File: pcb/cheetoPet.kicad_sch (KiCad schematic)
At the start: 46 parts, among them J1 SH1107 Display 128x128, P1 USB_C_Plug_USB2.0, SW1 B, SW2 X, SW3 A, SW4 POWER, SW5 RESET, SW6 BOOT, U1 DS3231M, U2 MPU-9250, U3 TP4056-42-ESOP8, U4 ESP32-C3-WROOM-02U, U5 ADS1115IDGS, U6 TPS63802DLAR, U7 AT24CS04-SSHM

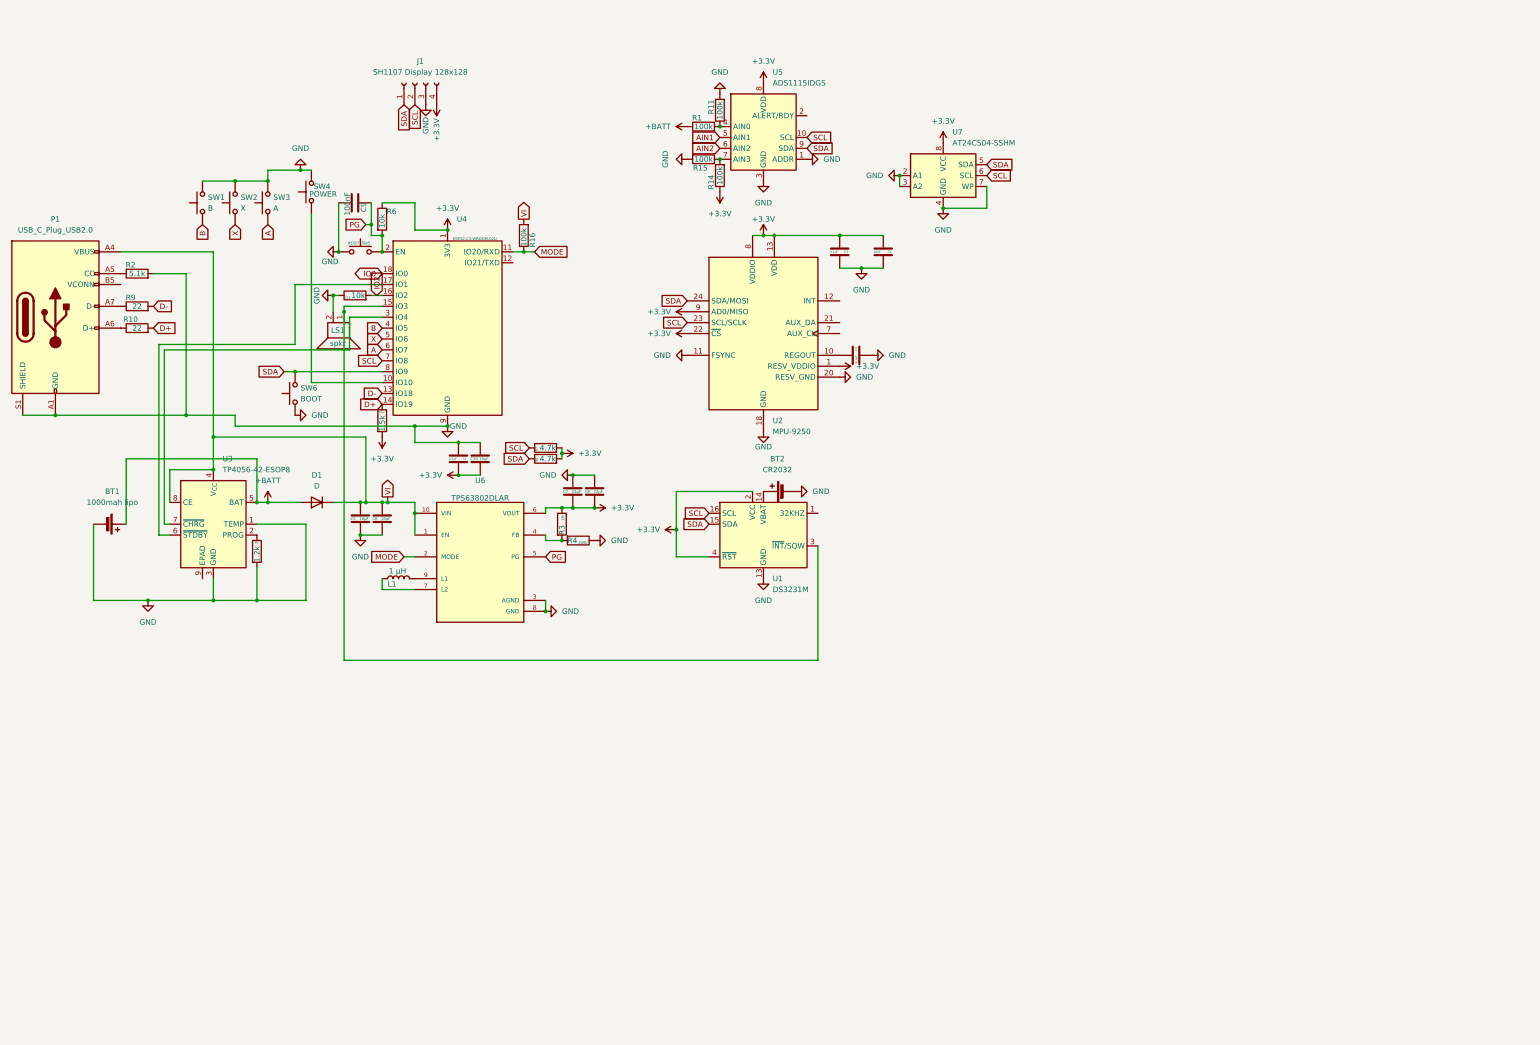
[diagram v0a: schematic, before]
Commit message: new pcb lol
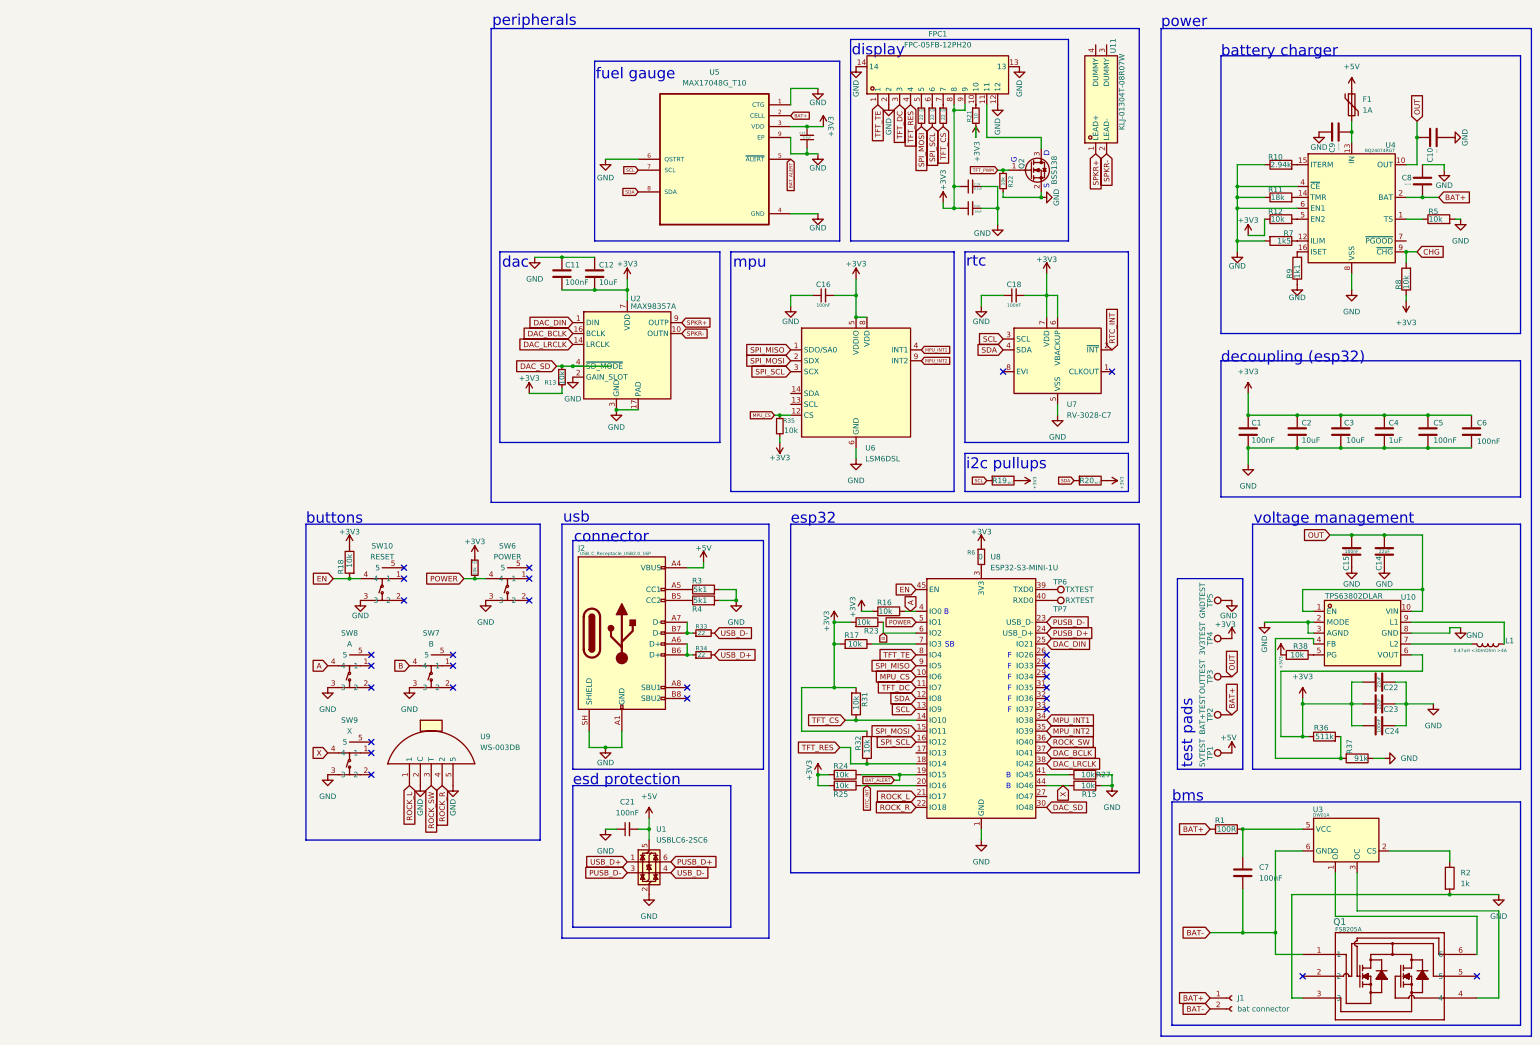
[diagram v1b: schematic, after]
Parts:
- removed BT1: 1000mah lipo, Connector_PinHeader_2.54mm:PinHeader_1x02_P2.54mm_Vertical, symbol Device:Battery_Cell
- removed BT2: CR2032, Connector_PinHeader_2.54mm:PinHeader_1x02_P2.54mm_Vertical, symbol Device:Battery_Cell
- removed D1: D, Diode_SMD:D_0805_2012Metric_Pad1.15x1.40mm_HandSolder, symbol Device:D
- removed J1: SH1107 Display 128x128, Connector_PinHeader_2.54mm:PinHeader_1x04_P2.54mm_Vertical, symbol Connector:Conn_01x04_Socket
- removed LS1: spkr, cheeto:PS1240_PassiveBuzzer_12.2x3.5mm, symbol Device:Speaker
- removed P1: USB_C_Plug_USB2.0, Connector_USB:USB_C_Receptacle_HRO_TYPE-C-31-M-12, symbol Connector:USB_C_Plug_USB2.0
- removed R13, R6: 10k, Resistor_SMD:R_0805_2012Metric_Pad1.20x1.40mm_HandSolder, symbol Device:R
- removed R14: 100k, Resistor_SMD:R_0805_2012Metric_Pad1.20x1.40mm_HandSolder, symbol Device:R
- removed SW1: B, Library:PushButton_SMD_3_4_2mm, symbol Switch:SW_Push
- removed SW2: X, Library:PushButton_SMD_3_4_2mm, symbol Switch:SW_Push
- removed SW3: A, Library:PushButton_SMD_3_4_2mm, symbol Switch:SW_Push
- removed SW4: POWER, cheeto:side switch, symbol Switch:SW_Push
- removed SW5: RESET, Library:PushButton_SMD_3_4_2mm, symbol Switch:SW_Push
- removed SW6: BOOT, Library:PushButton_SMD_3_4_2mm, symbol Switch:SW_Push
- removed U1: DS3231M, Package_SO:SOIC-16W_7.5x10.3mm_P1.27mm, symbol Timer_RTC:DS3231M
- removed U2: MPU-9250, Sensor_Motion:InvenSense_QFN-24_3x3mm_P0.4mm, symbol Sensor_Motion:MPU-9250
- removed U3: TP4056-42-ESOP8, Package_SO:SOIC-8-1EP_3.9x4.9mm_P1.27mm_EP2.41x3.3mm_ThermalVias, symbol Battery_Management:TP4056-42-ESOP8
- removed U4: ESP32-C3-WROOM-02U, RF_Module:ESP32-C3-WROOM-02U, symbol RF_Module:ESP32-C3-WROOM-02U
- removed U5: ADS1115IDGS, Package_SO:TSSOP-10_3x3mm_P0.5mm, symbol Analog_ADC:ADS1115IDGS
- removed U6: TPS63802DLAR, cheeto:VREG_TPS63802DLAR, symbol cheeto:TPS63802DLAR
- removed U7: AT24CS04-SSHM, Package_SO:SOIC-8_3.9x4.9mm_P1.27mm, symbol Memory_EEPROM:AT24CS04-SSHM
- added C11: 100nF, Capacitor_SMD:C_0402_1005Metric, symbol Device:C
- added C12: 10uF, Capacitor_SMD:C_0603_1608Metric, symbol Device:C
- added C14, C22, C23: 22uF, Capacitor_SMD:C_0805_2012Metric, symbol Device:C
- added C15, C24: 100nF, Capacitor_SMD:C_0603_1608Metric, symbol Device:C
- added C16, C18, C21: 100nF, Capacitor_SMD:C_0603_1608Metric, symbol Device:C_Small
- added C17, C19: 0.1uF, Capacitor_SMD:C_0402_1005Metric, symbol Device:C_Small
- added C20: 10uF, Capacitor_SMD:C_0603_1608Metric, symbol Device:C_Small
- added F1: 1A, Fuse:Fuse_1812_4532Metric, symbol Device:Polyfuse
- added FPC1: FPC-05FB-12PH20, EasyEDA:FPC-SMD_12P-P0.50_XUNPU_FPC-05FB-12PH20, symbol EasyEDA:FPC-05FB-12PH20
- added J1: bat connector, Connector_PinHeader_2.00mm:PinHeader_1x02_P2.00mm_Vertical, symbol Connector:Conn_01x02_Socket
- added J2: USB_C_Receptacle_USB2.0_16P, Connector_USB:USB_C_Receptacle_G-Switch_GT-USB-7010ASV, symbol Connector:USB_C_Receptacle_USB2.0_16P
- added Q1: FS8205A, footprints:SOT-23-6L_TCP, symbol 2026-06-26_17-03-40:FS8205A
- added Q2: BSS138, Package_TO_SOT_SMD:SOT-23, symbol Transistor_FET:BSS138
- added R13, R22, R26, R35: 10k, Resistor_SMD:R_0402_1005Metric, symbol Device:R_Small
- added R17, R18, R23, R24, R25, R27, R31, R32, R38: 10k, Resistor_SMD:R_0402_1005Metric, symbol Device:R
- added R19, R20: 4k7, Resistor_SMD:R_0402_1005Metric, symbol Device:R
- added R21: 10, Resistor_SMD:R_0402_1005Metric, symbol Device:R_Small
- added R28, R29, R30, R33, R34: 22, Resistor_SMD:R_0402_1005Metric, symbol Device:R_Small
- added R36: 511k, Resistor_SMD:R_0402_1005Metric, symbol Device:R
- added R37: 91k, Resistor_SMD:R_0402_1005Metric, symbol Device:R
- added R6: 0, Resistor_SMD:R_0402_1005Metric, symbol Device:R_Small
- added SW10: RESET, EasyEDA:SW-SMD_5P-L4.2-W2.8-P1.60-LS4.6-TR, symbol EasyEDA:KMR223GLFG
- added SW6: POWER, EasyEDA:SW-SMD_5P-L4.2-W2.8-P1.60-LS4.6-TR, symbol EasyEDA:KMR223GLFG
- added SW7: B, EasyEDA:SW-SMD_5P-L4.2-W2.8-P1.60-LS4.6-TR, symbol EasyEDA:KMR223GLFG
- added SW8: A, EasyEDA:SW-SMD_5P-L4.2-W2.8-P1.60-LS4.6-TR, symbol EasyEDA:KMR223GLFG
- added SW9: X, EasyEDA:SW-SMD_5P-L4.2-W2.8-P1.60-LS4.6-TR, symbol EasyEDA:KMR223GLFG
- added TP1: 5VTEST, TestPoint:TestPoint_Pad_1.5x1.5mm, symbol Connector:TestPoint
- added TP2: BAT+TEST, TestPoint:TestPoint_Pad_1.5x1.5mm, symbol Connector:TestPoint
- added TP3: OUTTEST, TestPoint:TestPoint_Pad_1.5x1.5mm, symbol Connector:TestPoint
- added TP4: 3V3TEST, TestPoint:TestPoint_Pad_1.5x1.5mm, symbol Connector:TestPoint
- added TP5: GNDTEST, TestPoint:TestPoint_Pad_1.5x1.5mm, symbol Connector:TestPoint
- added TP6: TXTEST, TestPoint:TestPoint_Pad_1.5x1.5mm, symbol Connector:TestPoint
- added TP7: RXTEST, TestPoint:TestPoint_Pad_1.5x1.5mm, symbol Connector:TestPoint
- added U1: USBLC6-2SC6, Package_TO_SOT_SMD:SOT-23-6, symbol Power_Protection:USBLC6-2SC6
- added U10: TPS63802DLAR, EasyEDA:VSON-10_L3.0-W2.0-P0.50-TL, symbol EasyEDA:TPS63802DLAR
- added U11: KLJ-01304T-08R07W, EasyEDA:BUZ-SMD_4P-L13.0-W13.0-P11.4-BL, symbol EasyEDA:KLJ-01304T-08R07W
- added U2: MAX98357A, Package_DFN_QFN:TQFN-16-1EP_3x3mm_P0.5mm_EP1.23x1.23mm, symbol Audio:MAX98357A
- added U3: DW01A, Package_TO_SOT_SMD:SOT-23-6, symbol Battery_Management:DW01A
- added U4: BQ24074RGT, Package_DFN_QFN:VQFN-16-1EP_3x3mm_P0.5mm_EP1.6x1.6mm, symbol Battery_Management:BQ24074RGT
- added U5: MAX17048G_T10, MAX17048G_T10:SON50P200X200X80-9N, symbol MAX17048G_T10:MAX17048G_T10
- added U6: LSM6DSL, Package_LGA:LGA-14_3x2.5mm_P0.5mm_LayoutBorder3x4y, symbol Sensor_Motion:LSM6DSL
- added U7: RV-3028-C7, Package_SON:MicroCrystal_C7_SON-8_1.5x3.2mm_P0.9mm, symbol Timer_RTC:RV-3028-C7
- added U8: ESP32-S3-MINI-1U, RF_Module:ESP32-S2-MINI-1U, symbol RF_Module:ESP32-S3-MINI-1U
- added U9: WS-003DB, EasyEDA:SW-SMD_WS-003DB, symbol EasyEDA:WS-003DB
- C1: value 0.1µF -> 100nF; footprint Capacitor_SMD:C_0805_2012Metric_Pad1.18x1.45mm_HandSolder -> Capacitor_SMD:C_0402_1005Metric
- C10: value 10µF -> 22uF; footprint Capacitor_SMD:C_0805_2012Metric_Pad1.18x1.45mm_HandSolder -> Capacitor_SMD:C_0805_2012Metric
- C2: value 0.1µf -> 10uF; footprint Capacitor_SMD:C_0805_2012Metric_Pad1.18x1.45mm_HandSolder -> Capacitor_SMD:C_0603_1608Metric
- C3: value 0.1uF -> 10uF; footprint Capacitor_SMD:C_0805_2012Metric_Pad1.18x1.45mm_HandSolder -> Capacitor_SMD:C_0603_1608Metric
- C4: value 10uF -> 1uF; footprint Capacitor_SMD:C_0805_2012Metric_Pad1.18x1.45mm_HandSolder -> Capacitor_SMD:C_0402_1005Metric
- C5, C6: value 10µF -> 100nF; footprint Capacitor_SMD:C_0805_2012Metric_Pad1.18x1.45mm_HandSolder -> Capacitor_SMD:C_0402_1005Metric
- C7: value 22µF -> 100nF; footprint Capacitor_SMD:C_0805_2012Metric_Pad1.18x1.45mm_HandSolder -> Capacitor_SMD:C_0402_1005Metric
- C8: value 22µF -> 10uF X5R; footprint Capacitor_SMD:C_0805_2012Metric_Pad1.18x1.45mm_HandSolder -> Capacitor_SMD:C_0603_1608Metric
- C9: value 100nF -> 10uF X5R; footprint Capacitor_SMD:C_0603_1608Metric_Pad1.08x0.95mm_HandSolder -> Capacitor_SMD:C_0603_1608Metric
- L1: value 1 µH -> 0.47uH <30mOhm >4A; footprint Inductor_SMD:L_Changjiang_FXL0420 -> EasyEDA:L1008
- R1: value 100k -> 100R; footprint Resistor_SMD:R_0805_2012Metric_Pad1.20x1.40mm_HandSolder -> Resistor_SMD:R_0402_1005Metric
- R10: value 22 -> 2.94k; footprint Resistor_SMD:R_0805_2012Metric_Pad1.20x1.40mm_HandSolder -> Resistor_SMD:R_0402_1005Metric
- R11: value 100k -> 18k; footprint Resistor_SMD:R_0805_2012Metric_Pad1.20x1.40mm_HandSolder -> Resistor_SMD:R_0402_1005Metric
- R12: value 1.5k -> 10k; footprint Resistor_SMD:R_0805_2012Metric_Pad1.20x1.40mm_HandSolder -> Resistor_SMD:R_0402_1005Metric
- R15, R16: value 100k -> 10k; footprint Resistor_SMD:R_0805_2012Metric_Pad1.20x1.40mm_HandSolder -> Resistor_SMD:R_0402_1005Metric
- R2: value 5.1k -> 1k; footprint Resistor_SMD:R_0805_2012Metric_Pad1.20x1.40mm_HandSolder -> Resistor_SMD:R_0402_1005Metric
- R3: value 1M -> 5k1; footprint Resistor_SMD:R_1206_3216Metric_Pad1.30x1.75mm_HandSolder -> Resistor_SMD:R_0402_1005Metric
- R4: value 309k -> 5k1; footprint Resistor_SMD:R_0402_1005Metric_Pad0.72x0.64mm_HandSolder -> Resistor_SMD:R_0402_1005Metric
- R5: value 1.2k -> 10k; footprint Resistor_SMD:R_0805_2012Metric_Pad1.20x1.40mm_HandSolder -> Resistor_SMD:R_0402_1005Metric
- R7: value 4.7k -> 1k5; footprint Resistor_SMD:R_0805_2012Metric_Pad1.20x1.40mm_HandSolder -> Resistor_SMD:R_0402_1005Metric
- R8: value 4.7k -> 10k; footprint Resistor_SMD:R_0805_2012Metric_Pad1.20x1.40mm_HandSolder -> Resistor_SMD:R_0402_1005Metric
- R9: value 22 -> 1k1; footprint Resistor_SMD:R_0805_2012Metric_Pad1.20x1.40mm_HandSolder -> Resistor_SMD:R_0402_1005Metric
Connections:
- net MODE is gone; now on net A: R16.1
- net VI is gone; now on net +3V3: C5.1, C6.1, R16.2
- net A: now also SW8.4, U8.4 (IO0)
- net B: now also R23.1, SW7.4, U8.6 (IO2)
- net GND: now also C1.2, C10.2, R10.1, R11.1, R3.2, R4.2, R7.2, R9.1, C11.1, C12.1, C14.2, C15.2, C16.1, C17.1, C18.1, C19.2, C20.2, C21.1, C22.2, C23.2, C24.2, FPC1.12, FPC1.13, FPC1.14, FPC1.2, J2.A1 (GND), J2.A12 (GND), J2.B1 (GND), J2.B12 (GND), J2.SH (SHIELD), Q1.3, Q2.2 (S), R22.2, R27.2, R37.1, SW10.3, SW6.3, SW7.3, SW8.3, SW9.3, TP5.1, U1.2 (GND), U10.2 (MODE), U10.3 (AGND), U10.8 (GND), U2.11 (GND), U2.15 (GND), U2.17 (PAD), U2.2 (GAIN_SLOT), U2.3 (GND), U4.17 (VSS), U4.4 (~{CE}), U4.6 (EN1), U4.8 (VSS), U5.1 (CTG), U5.4 (GND), U5.6 (QSTRT), U5.9 (EP), U6.6 (GND), U6.7 (GND), U7.5 (VSS), U8.1 (GND), U8.2 (GND), U8.42 (GND), U8.43 (GND), U8.46 (GND), U8.47 (GND), U8.48 (GND), U8.49 (GND), U8.50 (GND), U8.51 (GND), U8.52 (GND), U8.53 (GND), U8.54 (GND), U8.55 (GND), U8.56 (GND), U8.57 (GND), U8.58 (GND), U8.59 (GND), U8.60 (GND), U8.61 (GND), U8.62 (GND), U8.63 (GND), U8.64 (GND), U8.65 (GND), U9.2 (C), U9.5; no longer C1.1, C10.1, C7.1, R11.2, R4.1
- net SCL: now also R19.2, U5.7 (SCL), U7.3 (SCL), U8.13 (IO9); no longer R7.1
- net SDA: now also R20.2, U5.8 (SDA), U7.4 (SDA), U8.12 (IO8); no longer R8.1
- net X: now also R15.1, SW9.4, U8.44 (IO46)
- net +3V3: now reaches C2.1
- net +3V3: now also C1.1, C3.1, C4.1, R12.1, R8.1, C11.2, C12.2, C16.2, C17.2, C18.2, C19.1, C20.1, C22.1, C23.1, C24.1, FPC1.8, FPC1.9, R13.2, R17.2, R18.1, R19.1, R20.1, R21.2, R23.2, R24.2, R25.2, R26.1, R31.2, R32.2, R35.2, R36.1, R38.2, R6.1, TP4.1, U10.6 (VOUT), U2.7 (VDD), U2.8 (VDD), U5.3 (VDD), U6.5 (VDDIO), U6.8 (VDD), U7.6 (VBACKUP), U7.7 (VDD)
- net at R2.1: now also U3.2 (CS)
- net at R1.2: now also C7.1, U3.5 (VCC); no longer R11.1
- net at L1.1: now also U10.7 (L2)
- net at L1.2: now also U10.9 (L1)
- net at R5.1: now also U4.1 (TS)
- removed net +3.3V: C1.2, C10.2, C3.1, C4.1, C7.2, C8.2, R12.2, R3.1, R7.2, R8.2
- net +BATT renamed BAT+
- net BAT+: now also C8.2, J1.1 (Pin_1), TP2.1, U4.2 (BAT), U4.3 (BAT), U5.2 (CELL)
- net D+: no longer names the net of R10.2
- net D+: now also U4.15 (ITERM); no longer R12.1
- net D-: no longer names the net of R9.2
- net D-: now also U4.16 (ISET)
- net PG: no longer names the net of C9.2
- net PG: now also F1.2, U4.13 (IN)
- new net: R36.2, R37.2, U10.4 (FB)
- new net: FPC1.10, R21.1
- new net: FPC1.11, Q2.3 (D)
- new net: FPC1.5, R29.1
- new net: FPC1.6, R28.1
- new net: FPC1.7, R30.1
- new net: R7.1, U4.12 (ILIM)
- new net: R11.2, U4.14 (TMR)
- new net: R12.2, U4.5 (EN2)
- new net: TP6.1, U8.39 (TXD0)
- new net: R38.1, U10.5 (PG)
- new net: R17.1, U8.7 (IO3)
- new net: R27.1, U8.41 (IO45)
- new net: J2.A5 (CC1), R3.1
- new net: Q1.6, U3.1 (OD)
- new net: Q1.4, U3.3 (OC)
- new net: J2.A6 (D+), J2.B6 (D+), R34.1
- new net: J2.A7 (D-), J2.B7 (D-), R33.1
- new net: J2.B5 (CC2), R4.1
- new net: R6.2, U8.3 (3V3)
- new net: TP7.1, U8.40 (RXD0)
- new net +5V: C21.2, F1.1, J2.A4 (VBUS), J2.A9 (VBUS), J2.B4 (VBUS), J2.B9 (VBUS), TP1.1, U1.5 (VBUS)
- new net BAT-: C7.2, J1.2 (Pin_2), Q1.1, U3.6 (GND)
- new net BAT_ALERT: R24.1, U5.5 (~{ALERT}), U8.19 (IO15)
- new net CHG: R8.2, U4.9 (~{CHG})
- new net DAC_BCLK: U2.16 (BCLK), U8.37 (IO41)
- new net DAC_DIN: U2.1 (DIN), U8.25 (IO21)
- new net DAC_LRCLK: U2.14 (LRCLK), U8.38 (IO42)
- new net DAC_SD: R13.1, U2.4 (~{SD_MODE}), U8.30 (IO48)
- new net EN: R18.2, SW10.4, U8.45 (EN)
- new net MPU_CS: R35.1, U6.12 (CS), U8.10 (IO6)
- new net MPU_INT1: U6.4 (INT1), U8.34 (IO38)
- new net MPU_INT2: U6.9 (INT2), U8.35 (IO39)
- new net OUT: C10.1, C14.1, C15.1, TP3.1, U10.1 (EN), U10.10 (VIN), U4.10 (OUT), U4.11 (OUT)
- new net POWER: R26.2, SW6.4, U8.5 (IO1)
- new net PUSB_D+: U1.6 (I/O1), U8.24 (USB_D+)
- new net PUSB_D-: U1.3 (I/O2), U8.23 (USB_D-)
- new net ROCK_L: U8.21 (IO17), U9.1
- new net ROCK_R: U8.22 (IO18), U9.4 (2)
- new net ROCK_SW: U8.36 (IO40), U9.3 (T)
- new net RTC_INT: R25.1, U7.2 (~{INT}), U8.20 (IO16)
- new net SPI_MISO: U6.1 (SDO/SA0), U8.9 (IO5)
- new net SPI_MOSI: R29.2, U6.2 (SDX), U8.15 (IO11)
- new net SPI_SCL: R28.2, U6.3 (SCX), U8.16 (IO12)
- new net SPKR+: U11.1 (LEAD+), U2.9 (OUTP)
- new net SPKR-: U11.2 (LEAD-), U2.10 (OUTN)
- new net TFT_CS: R30.2, R31.1, U8.14 (IO10)
- new net TFT_DC: FPC1.3, U8.11 (IO7)
- new net TFT_PWM: Q2.1 (G), R22.1
- new net TFT_RES: FPC1.4, R32.1, U8.18 (IO14)
- new net TFT_TE: FPC1.1, U8.8 (IO4)
- new net USB_D+: R34.2, U1.1 (I/O1)
- new net USB_D-: R33.2, U1.4 (I/O2)
- no-connect marks 0 -> 27
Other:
- note added: "B"
- note added: "D"
- note added: "F"
- note added: "G"
- note added: "S"
- note added: "SB"
- note added: "battery charger"
- note added: "bms"
- note added: "buttons"
- note added: "connector"
- note added: "dac"
- note added: "decoupling (esp32)"
- note added: "display"
- note added: "esd protection"
- note added: "esp32"
- note added: "fuel gauge"
- note added: "i2c pullups"
- note added: "mpu"
- note added: "peripherals"
- note added: "power"
- note added: "rtc"
- note added: "test pads"
- note added: "usb"
- note added: "voltage management"
- company: cheeto industries -> (none)
- title: cheetoPet -> (none)
